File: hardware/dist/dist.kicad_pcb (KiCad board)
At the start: 2 copper layers, 173 parts, among them J1 PJ301M, J10 Conn_02x08_Odd_Even, J2 PJ301M, J3 PJ301M, J4 PJ301M, J5 PJ301M, J6 PJ301M, J7 PJ301M, J8 PJ301M, Q1 BC547B, Q2 BC547B, Q3 BC547B, Q4 BC547B, Q5 BSP89, SW1 SW_SPDT, SW2 SW_SPDT, SW3 SW_SPDT, U1 TL072, U2 TL072, U3 TL072, U4 TL072, U5 TL072, U6 TL072, U7 TL072

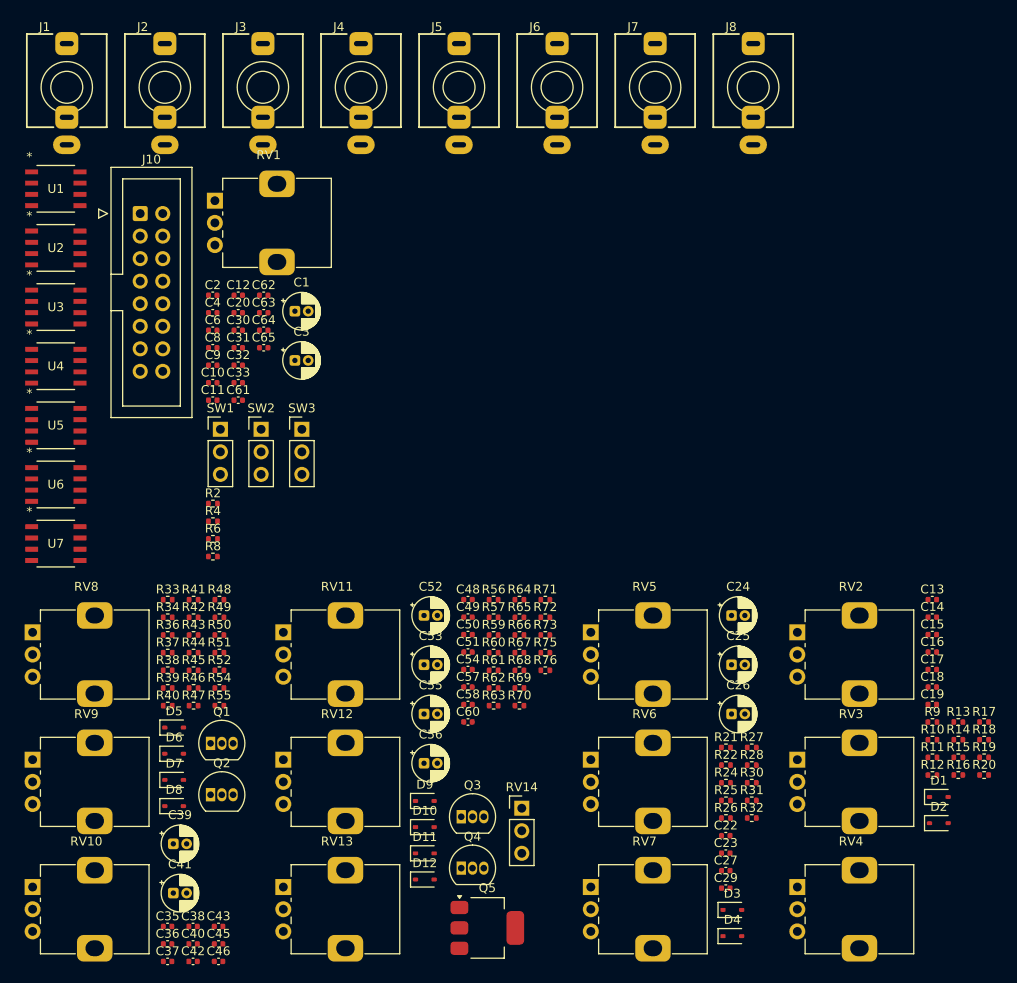
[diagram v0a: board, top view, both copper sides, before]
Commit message: finish pcb
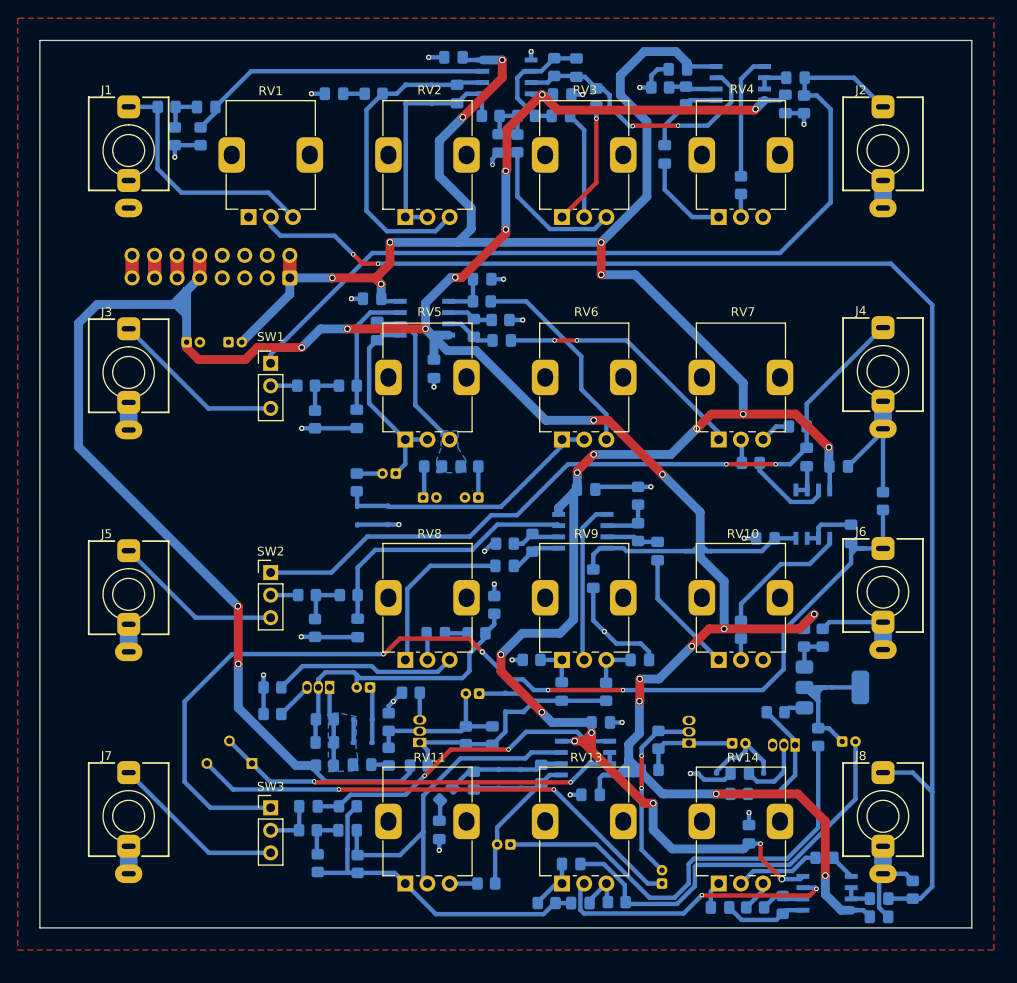
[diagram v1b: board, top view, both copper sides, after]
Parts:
- C1, C24, C25, C26, C3, C39, C41, C52, C53, C55, C56, D1, D10, D11, D12, D2, D3, D4, D5, D6, D7, D8, D9, J10, Q1, Q2, Q3, Q4, Q5, U1, U2, U3, U4, U5, U6, U7: moved to B.Cu
- C10, C11, C12, C13, C14, C15, C16, C17, C18, C19, C2, C20, C22, C23, C27, C29, C30, C31, C32, C33, C35, C36, C37, C38, C4, C40, C42, C43, C45, C46, C48, C49, C50, C51, C54, C57, C58, C6, C60, C61, C62, C63, C64, C65, C8, C9: footprint Capacitor_SMD:C_0402_1005Metric -> Capacitor_SMD:C_0805_2012Metric_Pad1.18x1.45mm_HandSolder; moved to B.Cu
- R10, R11, R12, R13, R14, R15, R16, R17, R18, R19, R2, R20, R21, R22, R24, R25, R26, R27, R28, R30, R31, R32, R33, R34, R36, R37, R38, R39, R4, R40, R41, R42, R43, R44, R45, R46, R47, R48, R49, R50, R51, R52, R54, R55, R56, R57, R59, R6, R60, R61, R62, R63, R65, R66, R67, R68, R69, R70, R71, R72, R73, R75, R76, R8, R9: footprint Resistor_SMD:R_0402_1005Metric -> Resistor_SMD:R_0805_2012Metric_Pad1.20x1.40mm_HandSolder; moved to B.Cu
- R64: value 1M -> 2.2M; footprint Resistor_SMD:R_0402_1005Metric -> Resistor_SMD:R_0805_2012Metric_Pad1.20x1.40mm_HandSolder; moved to B.Cu
- RV12: footprint Potentiometer_THT:Potentiometer_Alps_RK09K_Single_Vertical -> 3362P-1-253LF:TRIM_3362P-1-253LF; moved to B.Cu
- RV14: footprint Connector_PinHeader_2.54mm:PinHeader_1x03_P2.54mm_Vertical -> Potentiometer_THT:Potentiometer_Alps_RK09K_Single_Vertical
- moved R9 110.7 mm to (29.3, 22.5)
- moved R10 109.1 mm to (30.2, 25.8), turned to 90 degrees
- moved R11 108.2 mm to (33.1, 25.8), turned to 90 degrees
- moved D2 101.8 mm to (56.2, 21.1), turned to -90 degrees
- moved J7 101.3 mm to (25.0, 102.4)
- moved R12 99.3 mm to (52.6, 21.0), turned to 180 degrees
- moved C13 98.9 mm to (33.7, 22.5)
- moved D1 97.7 mm to (59.1, 21.1), turned to 90 degrees
- moved C8 97.4 mm to (109.6, 111.7)
- moved C64 95.8 mm to (109.5, 113.8)
- moved U7 95.4 mm to (103.7, 111.1)
- moved C15 90.9 mm to (48.1, 21.0), turned to 180 degrees
- moved R17 88.3 mm to (73.0, 18.0), turned to -90 degrees
- moved R8 87.3 mm to (113.3, 110.7), turned to 90 degrees
- moved R15 87.2 mm to (69.8, 23.5)
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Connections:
- C35 pad 2: Net-(U4B-+) -> Net-(U5A-+)
- C52 pad 1: Net-(Q3-B) -> Net-(C52-Pad1)
- C52 pad 2: Net-(C52-Pad2) -> Net-(Q3-B)
- C6 pad 1: Net-(U5B--) -> Net-(U4B--)
- R36 pad 1: Net-(U4B-+) -> Net-(U5A-+)
- R37 pad 2: Net-(U4B--) -> Net-(U5A--)
- R38 pad 1: Net-(U4B--) -> Net-(U5A--)
- R44 pad 2: VDD -> +12V
- R48 pad 2: VDD -> +12V
- R52 pad 2: Net-(U5A--) -> Net-(U5B--)
- R54 pad 1: Net-(U5A--) -> Net-(U5B--)
- R65 pad 2: VDD -> +12V
- R66 pad 2: VDD -> +12V
- R69 pad 2: VDD -> +12V
- RV12 pad 3: Net-(C52-Pad2) -> Net-(C52-Pad1)
- RV9 pad 2: Net-(U5A-+) -> Net-(U5B-+)
- U4 pad 5: Net-(U4B-+) -> /FUZZ Circuit/OUT
- U4 pad 7: Net-(C36-Pad1) -> Net-(U4B--)
- U5 pad 1: Net-(C46-Pad1) -> Net-(C36-Pad1)
- U5 pad 5: /FUZZ Circuit/OUT -> Net-(U5B-+)
- U5 pad 7: Net-(U5B--) -> Net-(C46-Pad1)
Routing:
- net +12V: track 0.00 -> 387.0 mm, vias 0 -> 19
- net -12V: track 0.00 -> 273.5 mm, vias 0 -> 19
- net GND: track 0.00 -> 181.1 mm, vias 0 -> 28
- net /WRMERGLE_OUT: track 0.00 -> 156.8 mm, vias 0 -> 2
- net /FUZZ_OUT: track 0.00 -> 121.6 mm, vias 0 -> 4
- net /OD_OUT: track 0.00 -> 97.5 mm
- net /DIST_OUT: track 0.00 -> 83.3 mm, vias 0 -> 2
- net Net-(C52-Pad1): track 0.00 -> 56.9 mm, vias 0 -> 2
- net Net-(C55-Pad1): track 0.00 -> 50.9 mm
- net Net-(U6B--): track 0.00 -> 46.9 mm, vias 0 -> 2
- net Net-(C56-Pad2): track 0.00 -> 46.8 mm
- net Net-(U6A-+): track 0.00 -> 39.0 mm
- net Net-(U6B-+): track 0.00 -> 36.8 mm, vias 0 -> 2
- net Net-(D1-A): track 0.00 -> 36.8 mm
- net Net-(U1A-+): track 0.00 -> 34.8 mm
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- added copper zone on F.Cu, net GND
- added copper zone on B.Cu, net Net-(D5-K)
- added copper zone on B.Cu, net Net-(U3A--)
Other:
- board outline added: 105 x 100 mm
